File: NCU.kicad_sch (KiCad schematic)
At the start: 3 parts, among them J2 USB_C_Receptacle_USB2.0_14P

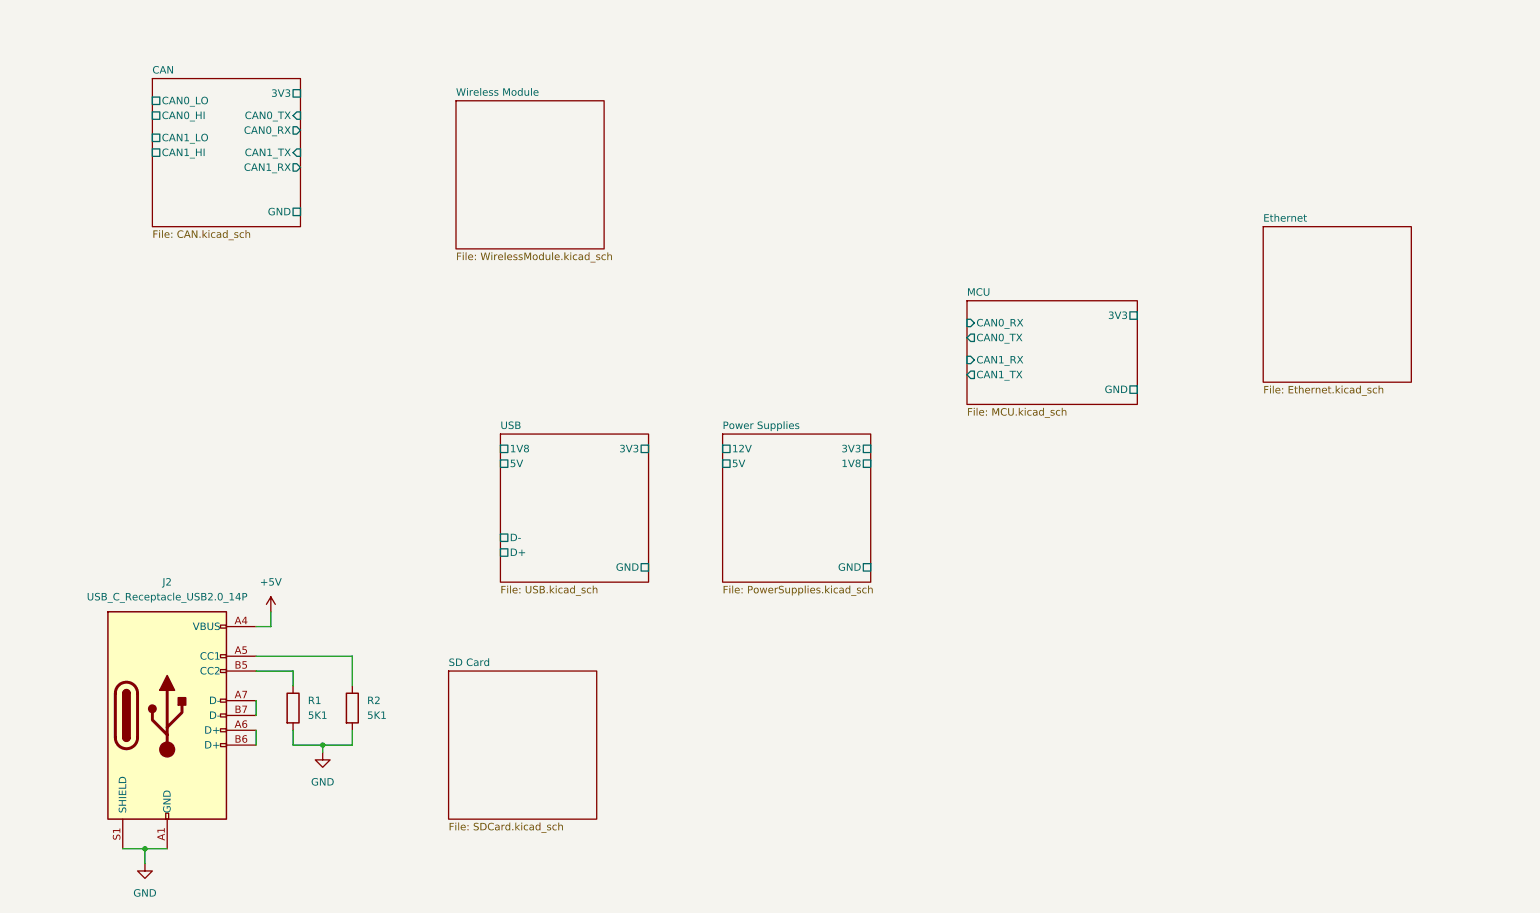
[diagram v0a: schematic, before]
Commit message: wip
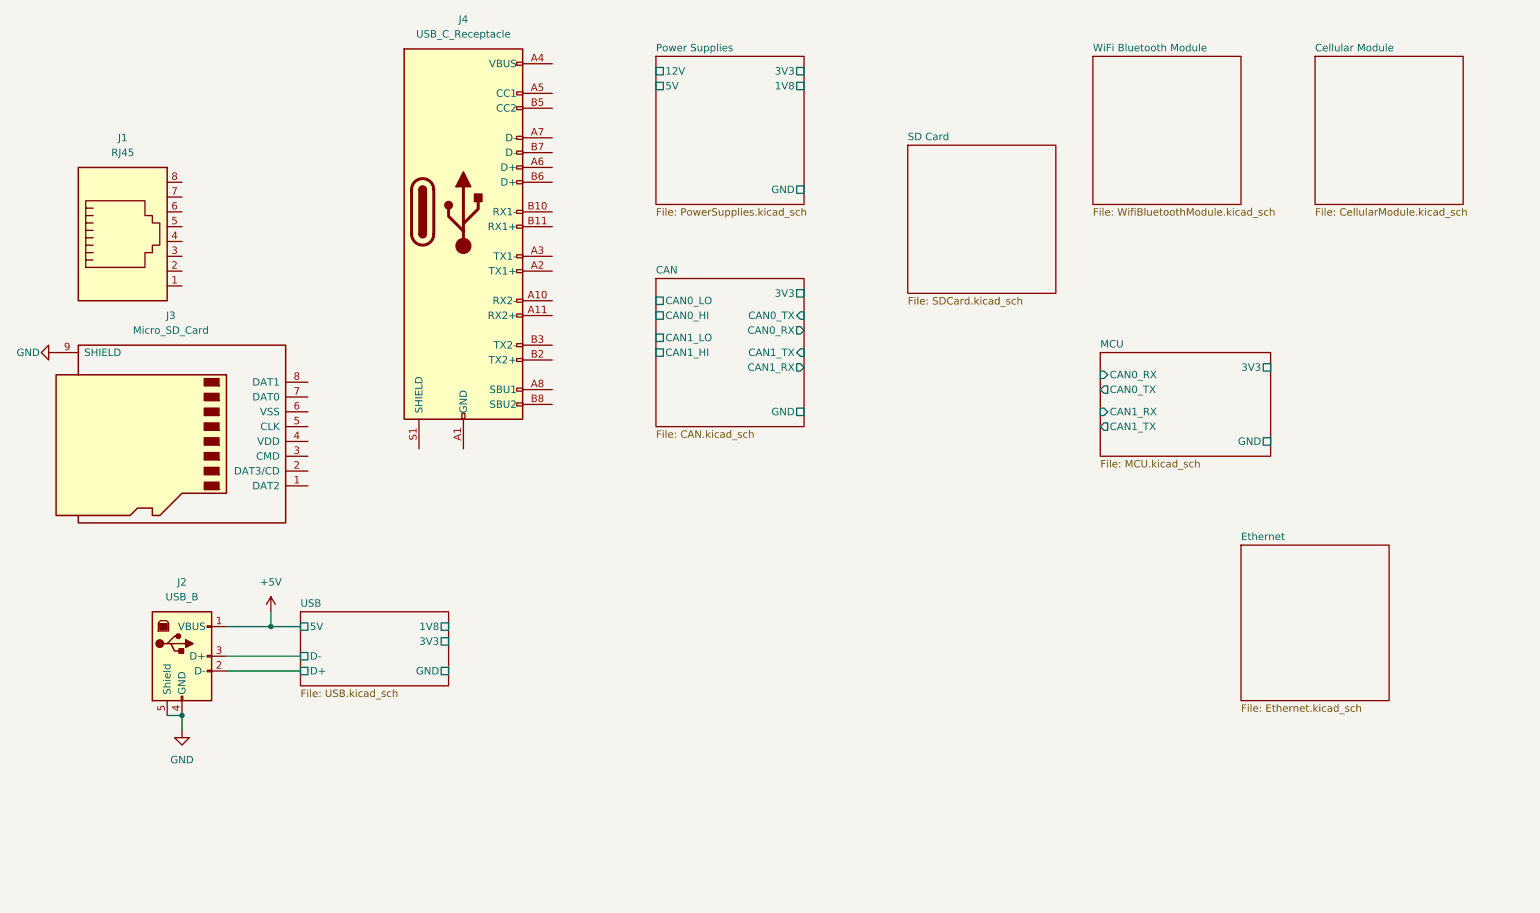
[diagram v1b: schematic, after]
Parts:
- removed J2: USB_C_Receptacle_USB2.0_14P, Connector_USB:USB_C_Receptacle_GCT_USB4110, symbol Connector:USB_C_Receptacle_USB2.0_14P
- removed R1, R2: 5K1, symbol Device:R
- added J1: RJ45, Connector_RJ:RJ45_Hanrun_HR911105A_Horizontal, symbol Connector:RJ45
- added J2: USB_B, symbol Connector:USB_B
- added J3: Micro_SD_Card, Connector_Card:microSD_HC_Molex_47219-2001, symbol Connector:Micro_SD_Card
- added J4: USB_C_Receptacle, symbol Connector:USB_C_Receptacle
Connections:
- net +5V: now also J2.1 (VBUS)
- net GND: now also J2.4 (GND), J2.5 (Shield), J3.9 (SHIELD)
- net USB/D+: now also J2.2 (D-)
- net USB/D-: now also J2.3 (D+)
- new net: J4.A1 (GND), J4.A12 (GND), J4.B1 (GND), J4.B12 (GND)
- new net: J4.A4 (VBUS), J4.A9 (VBUS), J4.B4 (VBUS), J4.B9 (VBUS)
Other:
- sheet Wireless Module renamed WiFi Bluetooth Module
- added sheet Cellular Module (CellularModule.kicad_sch)
- sheet WiFi Bluetooth Module: file WirelessModule.kicad_sch -> WifiBluetoothModule.kicad_sch
